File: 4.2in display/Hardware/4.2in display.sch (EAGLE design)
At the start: 41 parts, among them J2 MICRO-SD_CARD_SOCKETPUSH-PUSH, Q1 310mA/60V/1.6Ω, U2 3.3V, U4 23K640

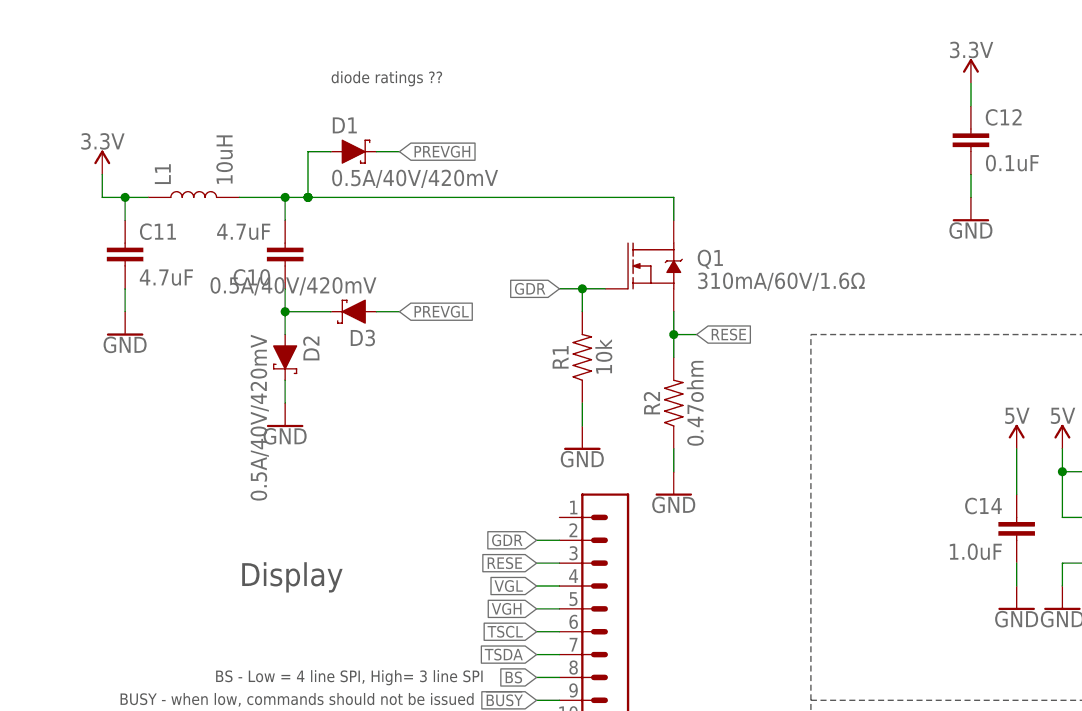
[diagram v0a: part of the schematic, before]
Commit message: asm
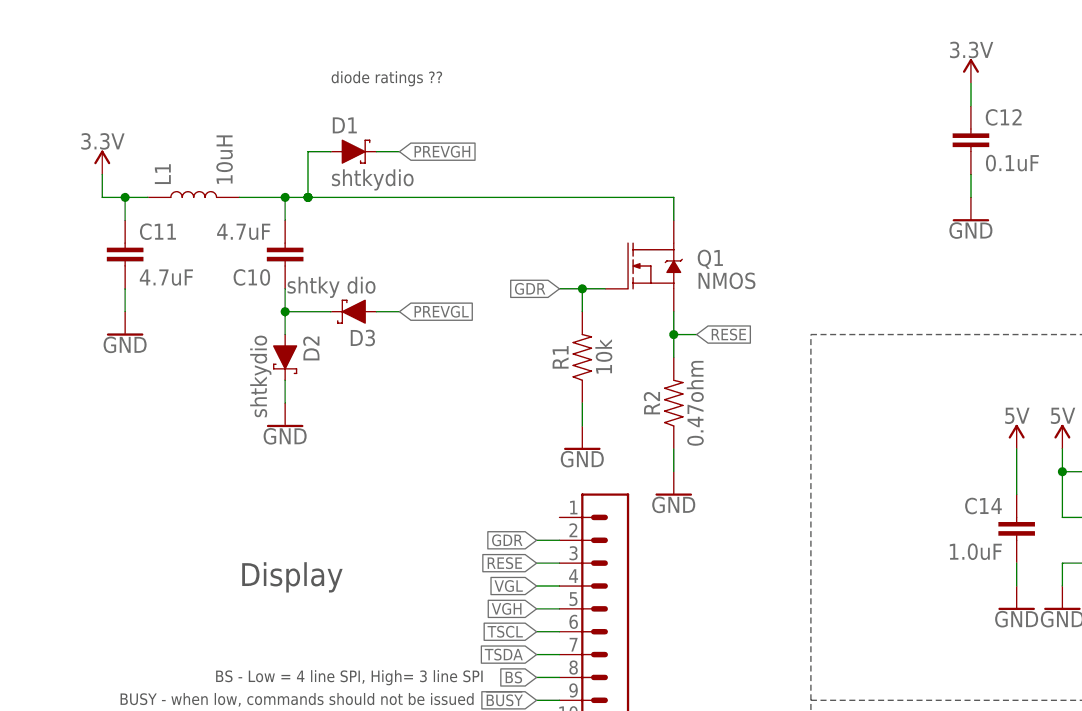
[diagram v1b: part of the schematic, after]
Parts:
- D1, D2: value 0.5A/40V/420mV -> shtkydio
- D3: value 0.5A/40V/420mV -> shtky dio
- Q1: value 310mA/60V/1.6Ω -> NMOS
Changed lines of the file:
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@@
 <?xml version="1.0" encoding="utf-8"?>
 <!DOCTYPE eagle SYSTEM "eagle.dtd">
-<eagle version="9.0.1">
+<eagle version="9.1.3">
 <drawing>
 <settings>
@@
 <part name="C8" library="SparkFun-Capacitors" deviceset="1.0UF" device="-0805-25V-10%" value="1.0uF"/>
 <part name="GND9" library="SparkFun-PowerSymbols" deviceset="GND" device=""/>
-<part name="Q1" library="SparkFun-DiscreteSemi" deviceset="MOSFET-NCH" device="-2N7002PW" value="310mA/60V/1.6Ω"/>
-<part name="D1" library="SparkFun-DiscreteSemi" deviceset="DIODE-SCHOTTKY" device="-PMEG4005EJ" value="0.5A/40V/420mV"/>
-<part name="D2" library="SparkFun-DiscreteSemi" deviceset="DIODE-SCHOTTKY" device="-PMEG4005EJ" value="0.5A/40V/420mV"/>
-<part name="D3" library="SparkFun-DiscreteSemi" deviceset="DIODE-SCHOTTKY" device="-PMEG4005EJ" value="0.5A/40V/420mV"/>
+<part name="Q1" library="SparkFun-DiscreteSemi" deviceset="MOSFET-NCH" device="-2N7002PW" value="NMOS"/>
+<part name="D1" library="SparkFun-DiscreteSemi" deviceset="DIODE-SCHOTTKY" device="-PMEG4005EJ" value="shtkydio"/>
+<part name="D2" library="SparkFun-DiscreteSemi" deviceset="DIODE-SCHOTTKY" device="-PMEG4005EJ" value="shtkydio"/>
+<part name="D3" library="SparkFun-DiscreteSemi" deviceset="DIODE-SCHOTTKY" device="-PMEG4005EJ" value="shtky dio"/>
 <part name="C9" library="SparkFun-Capacitors" deviceset="1.0UF" device="-0805-25V-10%" value="1.0uF"/>
 <part name="GND10" library="SparkFun-PowerSymbols" deviceset="GND" device=""/>

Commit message: Revert "asm"
This reverts commit 79dfb80ccaf4c70f6c8d653a0d6d0867a03f4c3a.
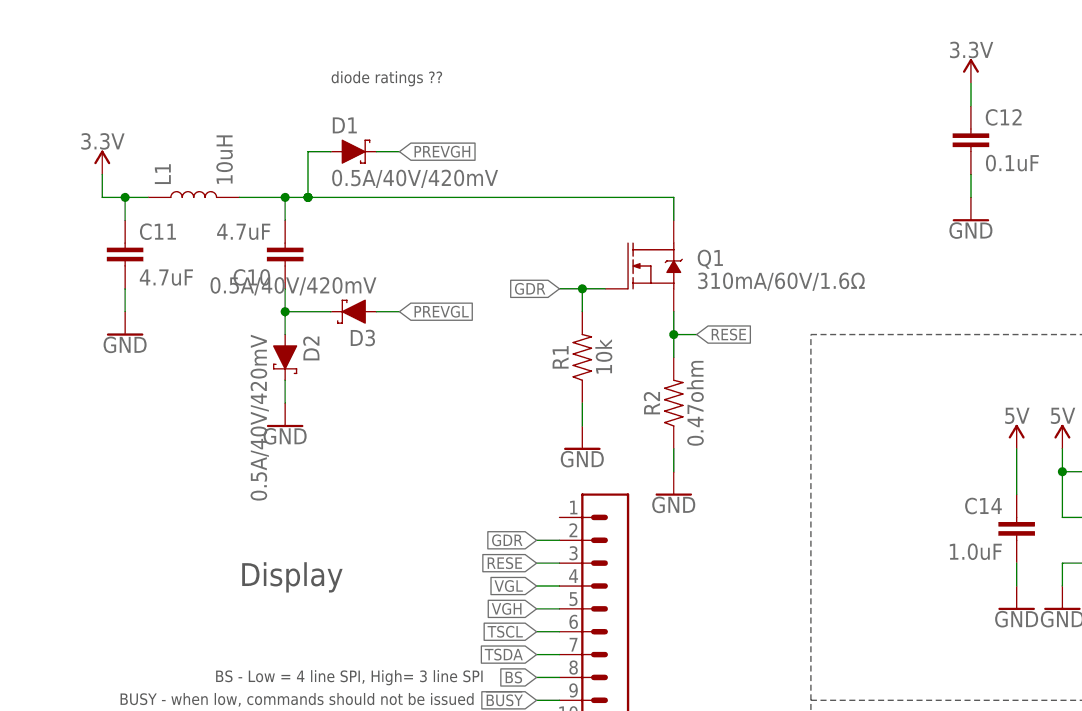
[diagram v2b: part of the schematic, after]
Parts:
- D1, D2: value shtkydio -> 0.5A/40V/420mV
- D3: value shtky dio -> 0.5A/40V/420mV
- Q1: value NMOS -> 310mA/60V/1.6Ω
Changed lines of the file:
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@@
 <?xml version="1.0" encoding="utf-8"?>
 <!DOCTYPE eagle SYSTEM "eagle.dtd">
-<eagle version="9.1.3">
+<eagle version="9.0.1">
 <drawing>
 <settings>
@@
 <part name="C8" library="SparkFun-Capacitors" deviceset="1.0UF" device="-0805-25V-10%" value="1.0uF"/>
 <part name="GND9" library="SparkFun-PowerSymbols" deviceset="GND" device=""/>
-<part name="Q1" library="SparkFun-DiscreteSemi" deviceset="MOSFET-NCH" device="-2N7002PW" value="NMOS"/>
-<part name="D1" library="SparkFun-DiscreteSemi" deviceset="DIODE-SCHOTTKY" device="-PMEG4005EJ" value="shtkydio"/>
-<part name="D2" library="SparkFun-DiscreteSemi" deviceset="DIODE-SCHOTTKY" device="-PMEG4005EJ" value="shtkydio"/>
-<part name="D3" library="SparkFun-DiscreteSemi" deviceset="DIODE-SCHOTTKY" device="-PMEG4005EJ" value="shtky dio"/>
+<part name="Q1" library="SparkFun-DiscreteSemi" deviceset="MOSFET-NCH" device="-2N7002PW" value="310mA/60V/1.6Ω"/>
+<part name="D1" library="SparkFun-DiscreteSemi" deviceset="DIODE-SCHOTTKY" device="-PMEG4005EJ" value="0.5A/40V/420mV"/>
+<part name="D2" library="SparkFun-DiscreteSemi" deviceset="DIODE-SCHOTTKY" device="-PMEG4005EJ" value="0.5A/40V/420mV"/>
+<part name="D3" library="SparkFun-DiscreteSemi" deviceset="DIODE-SCHOTTKY" device="-PMEG4005EJ" value="0.5A/40V/420mV"/>
 <part name="C9" library="SparkFun-Capacitors" deviceset="1.0UF" device="-0805-25V-10%" value="1.0uF"/>
 <part name="GND10" library="SparkFun-PowerSymbols" deviceset="GND" device=""/>
